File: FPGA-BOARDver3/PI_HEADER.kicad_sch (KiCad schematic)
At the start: 1 part, among them J9 Conn_02x20_Top_Bottom

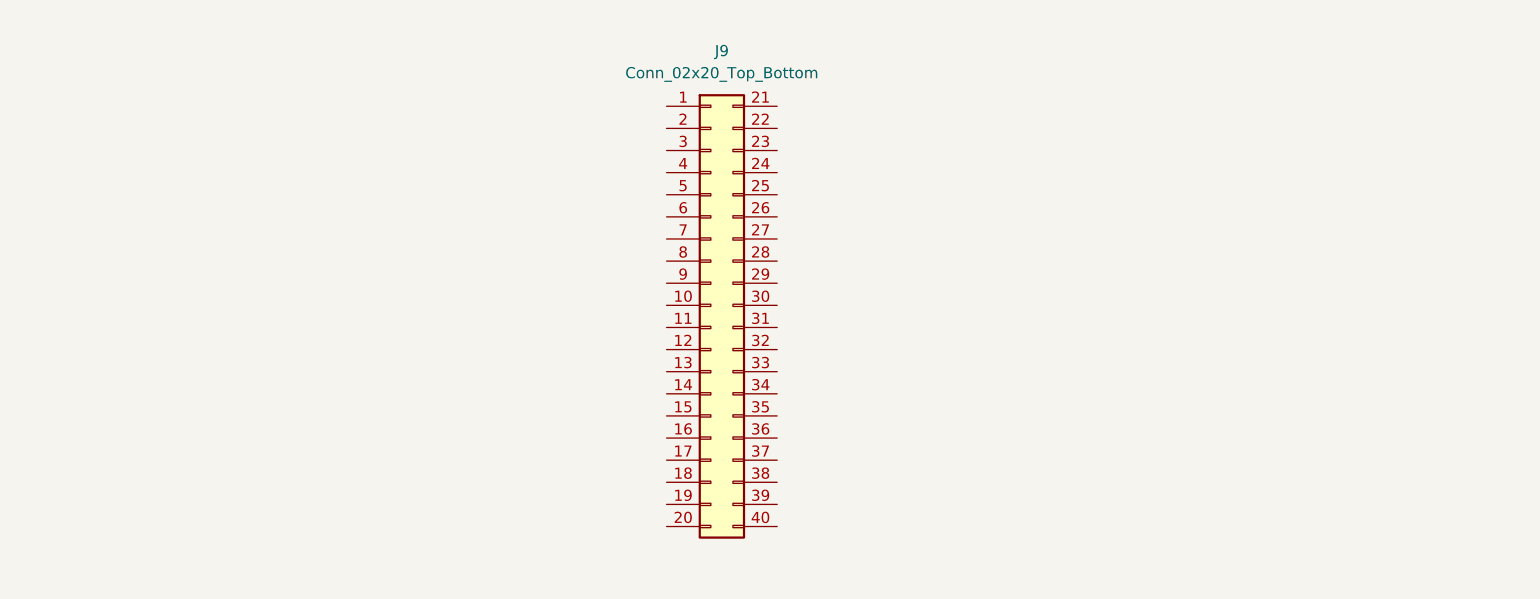
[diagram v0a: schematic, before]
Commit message: update
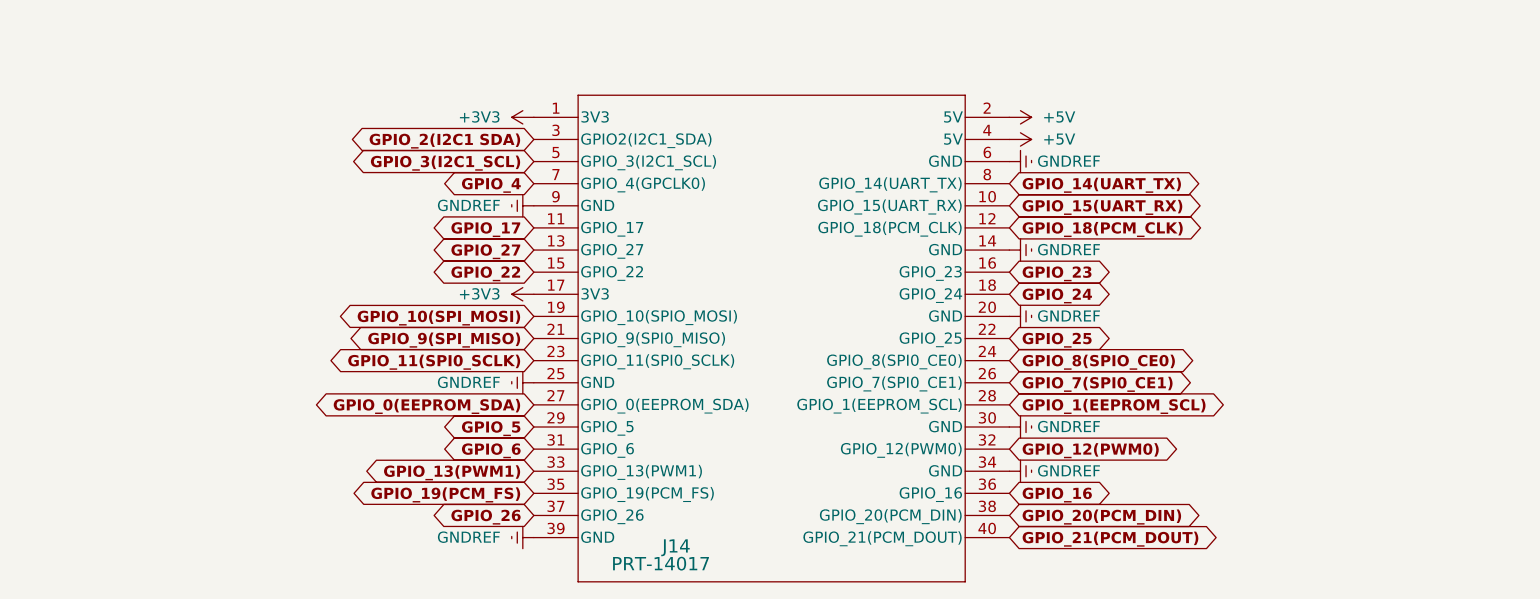
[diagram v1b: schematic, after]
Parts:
- removed J9: Conn_02x20_Top_Bottom, Connector_PinHeader_2.54mm:PinHeader_2x20_P2.54mm_Vertical, symbol Connector_Generic:Conn_02x20_Top_Bottom
- added J14: PRT-14017, footprints:CONN_PRT-14017_SPK, symbol PRT-14017:PRT-14017
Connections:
- new net +3V3: J14.1 (3V3), J14.17 (3V3)
- new net +5V: J14.2 (5V), J14.4 (5V)
- new net GNDREF: J14.14 (GND), J14.20 (GND), J14.25 (GND), J14.30 (GND), J14.34 (GND), J14.39 (GND), J14.6 (GND), J14.9 (GND)
- new net GPIO_0(EEPROM_SDA): J14.27 (GPIO_0(EEPROM_SDA))
- new net GPIO_1(EEPROM_SCL): J14.28 (GPIO_1(EEPROM_SCL))
- new net GPIO_10(SPI_MOSI): J14.19 (GPIO_10(SPIO_MOSI))
- new net GPIO_11(SPI0_SCLK): J14.23 (GPIO_11(SPI0_SCLK))
- new net GPIO_12(PWM0): J14.32 (GPIO_12(PWM0))
- new net GPIO_13(PWM1): J14.33 (GPIO_13(PWM1))
- new net GPIO_14(UART_TX): J14.8 (GPIO_14(UART_TX))
- new net GPIO_15(UART_RX): J14.10 (GPIO_15(UART_RX))
- new net GPIO_16: J14.36 (GPIO_16)
- new net GPIO_17: J14.11 (GPIO_17)
- new net GPIO_18(PCM_CLK): J14.12 (GPIO_18(PCM_CLK))
- new net GPIO_19(PCM_FS): J14.35 (GPIO_19(PCM_FS))
- new net GPIO_2(I2C1 SDA): J14.3 (GPIO2(I2C1_SDA))
- new net GPIO_20(PCM_DIN): J14.38 (GPIO_20(PCM_DIN))
- new net GPIO_21(PCM_DOUT): J14.40 (GPIO_21(PCM_DOUT))
- new net GPIO_22: J14.15 (GPIO_22)
- new net GPIO_23: J14.16 (GPIO_23)
- new net GPIO_24: J14.18 (GPIO_24)
- new net GPIO_25: J14.22 (GPIO_25)
- new net GPIO_26: J14.37 (GPIO_26)
- new net GPIO_27: J14.13 (GPIO_27)
- new net GPIO_3(I2C1_SCL): J14.5 (GPIO_3(I2C1_SCL))
- new net GPIO_4: J14.7 (GPIO_4(GPCLK0))
- new net GPIO_5: J14.29 (GPIO_5)
- new net GPIO_6: J14.31 (GPIO_6)
- new net GPIO_7(SPI0_CE1): J14.26 (GPIO_7(SPI0_CE1))
- new net GPIO_8(SPIO_CE0): J14.24 (GPIO_8(SPI0_CE0))
- new net GPIO_9(SPI_MISO): J14.21 (GPIO_9(SPI0_MISO))

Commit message: schematic pages for review
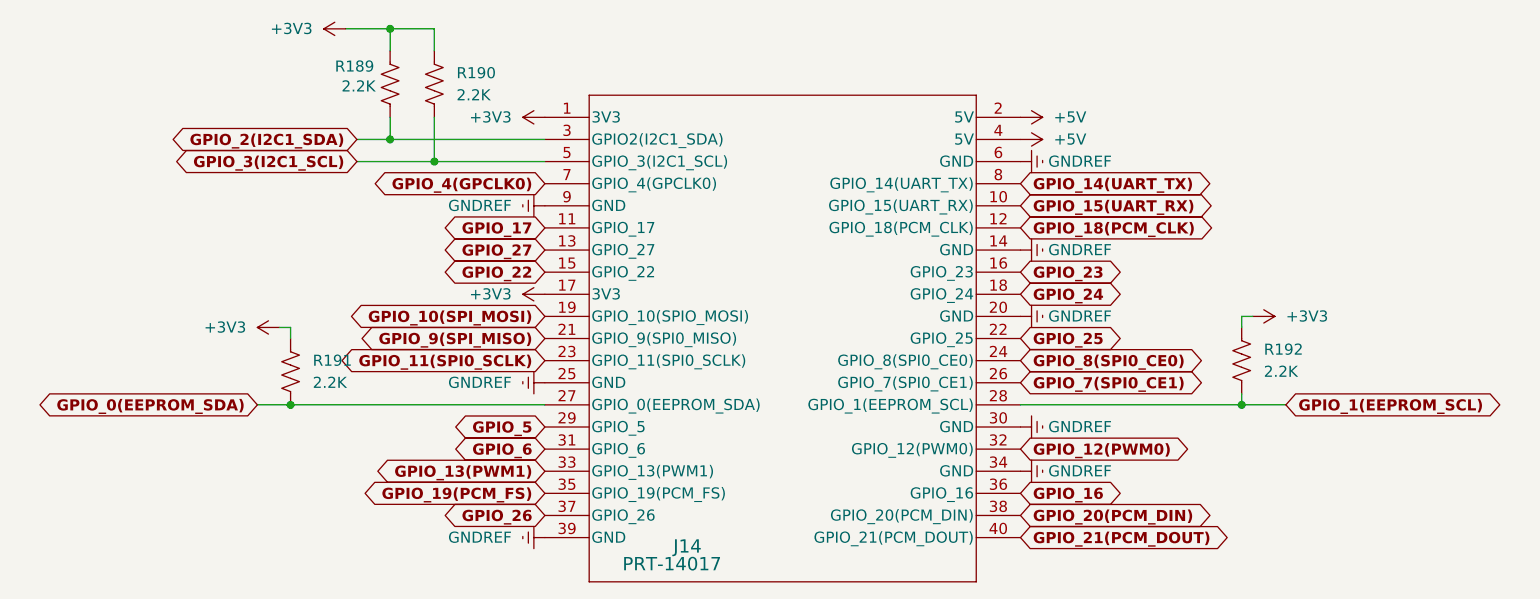
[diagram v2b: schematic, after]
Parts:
- added R189, R190, R191, R192: 2.2K, footprints:R_0402, symbol Device:R_US
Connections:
- net +3V3: now also R189.2, R190.2, R191.2, R192.2
- net GPIO_0(EEPROM_SDA): now also R191.1
- net GPIO_1(EEPROM_SCL): now also R192.1
- net GPIO_3(I2C1_SCL): now also R190.1
- net GPIO_2(I2C1 SDA) renamed GPIO_2(I2C1_SDA)
- net GPIO_2(I2C1_SDA): now also R189.1
- net GPIO_4 renamed GPIO_4(GPCLK0)
- net GPIO_8(SPIO_CE0) renamed GPIO_8(SPI0_CE0)
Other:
- moved on the sheet: J14
